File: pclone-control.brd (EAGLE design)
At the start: 72.4 x 68.6 mm, 20 parts

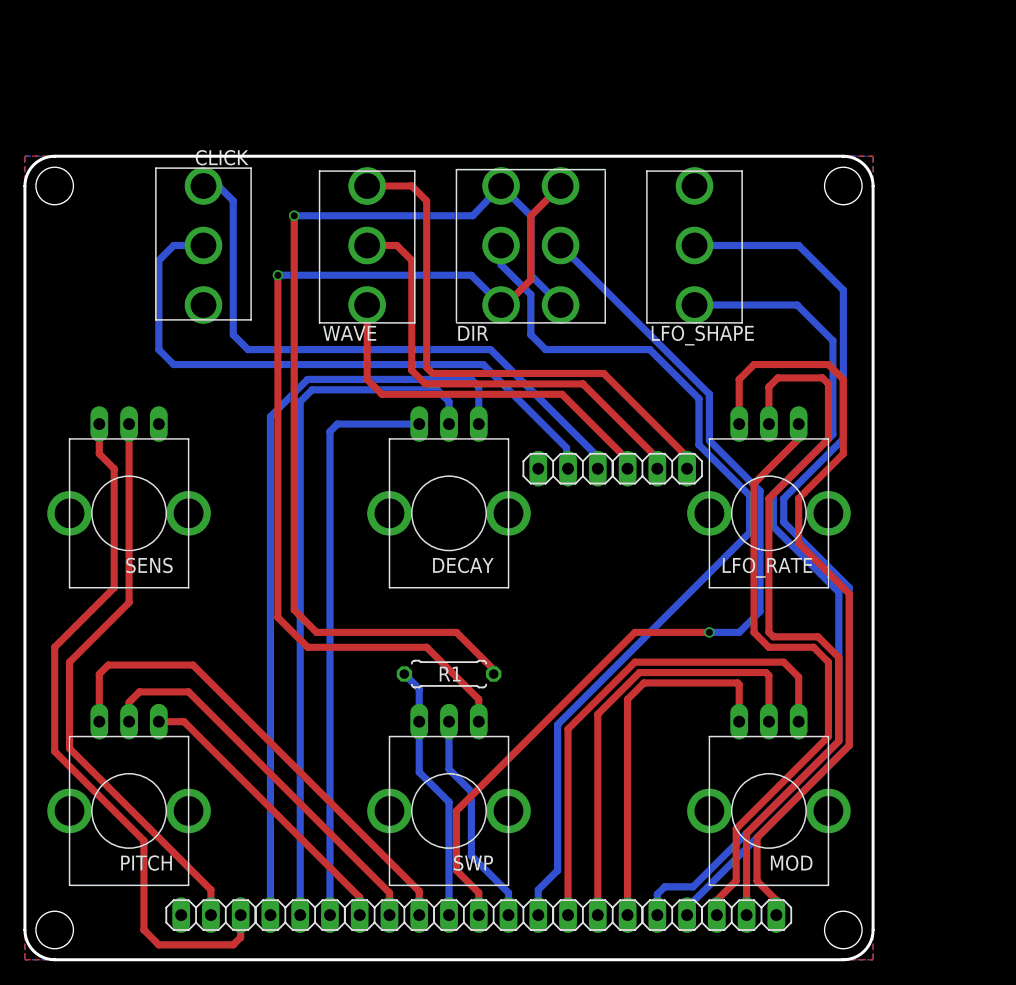
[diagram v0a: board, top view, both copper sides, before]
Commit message: work in progress
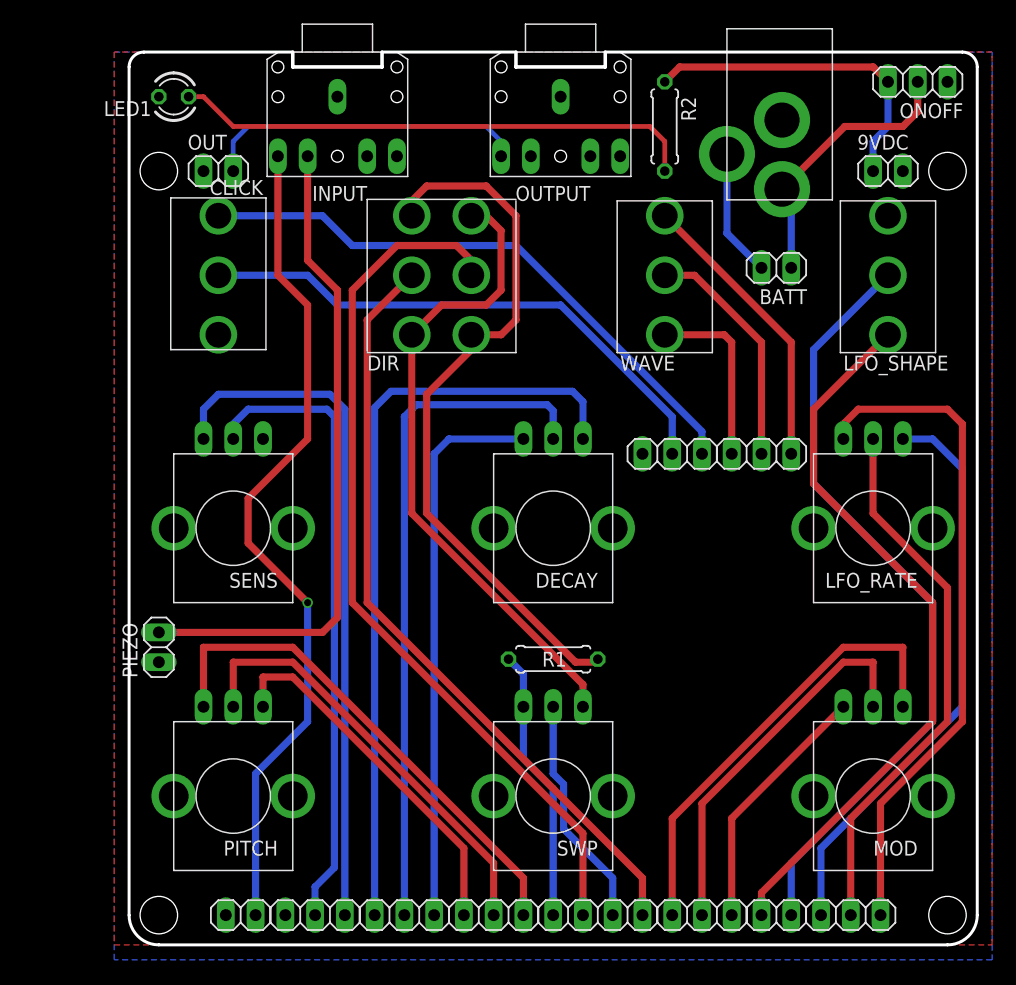
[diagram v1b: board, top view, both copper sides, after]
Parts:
- added 9VDC, BATT, IN, OUT, PIEZO: (no value), pinhead:1X02
- added INPUT, OUTPUT: TRUCONNECTJACK, jason_eagle6:TRUCONNECTJACK
- added LED1: (no value), led:LED3MM
- added ONOFF: (no value), pinhead:1X03
- added R2: 4k7, rcl:0207/7
- added U$4: 2.1MMJACKTHM, adafruit:PJ-102A
- moved WAVE 25.5 mm to (54.6, 58.4)
- moved LFO_SHAPE 16.7 mm to (73.7, 58.4)
- moved DECAY 8.98 mm to (45.1, 36.8)
- moved J8 8.98 mm to (55.2, 43.2)
- moved J9 8.98 mm to (62.9, 43.2)
- moved LFO_RATE 8.98 mm to (72.4, 36.8)
- moved MOD 8.98 mm to (72.4, 14.0)
- moved PITCH 8.98 mm to (17.8, 14.0)
- moved R1 8.98 mm to (45.1, 25.7)
- moved SENS 8.98 mm to (17.8, 36.8)
- moved SWP 8.98 mm to (45.1, 14.0)
- moved J6 8.89 mm to (64.1, 3.81)
- moved J3 8.89 mm to (40.0, 3.81)
- moved J1 8.89 mm to (24.8, 3.81)
- moved J4 8.89 mm to (48.9, 3.81)
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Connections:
- new net N$15: BATT.1, ONOFF.2, U$4.TIP
- new net N$29: BATT.2, U$4.RING_SW
- new net N$30: 9VDC.1, ONOFF.3, R2.1
- new net N$31: LED1.A, R2.2
- new net N$32: OUT.2, OUTPUT.TIP
- new net N$33: INPUT.TIP_NC, PIEZO.2
- new net N$34: IN.2, INPUT.TIP
- net GND: now also 9VDC.2, IN.1, INPUT.RING, INPUT.RING_NC, INPUT.SLEEVE, LED1.K, OUT.1, OUTPUT.RING, OUTPUT.RING_NC, OUTPUT.SLEEVE, PIEZO.1, U$4.RING
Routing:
- net N$34: track 0.00 -> 71.9 mm, vias 0 -> 1
- net N$33: track 0.00 -> 56.2 mm
- net N$31: track 0.00 -> 44.8 mm
- net N$3: track 83.7 -> 55.1 mm, vias 1 -> 0
- net N$30: track 0.00 -> 28.2 mm
- net N$32: track 0.00 -> 27.7 mm
- net N$15: track 0.00 -> 23.9 mm
- net N$2: track 84.2 -> 61.8 mm, vias 1 -> 0
- net N$8: track 46.2 -> 24.8 mm
- net N$9: track 38.7 -> 20.1 mm
- net N$26: track 64.2 -> 46.7 mm
- net N$7: track 32.2 -> 15.5 mm
- net N$4: track 78.6 -> 65.9 mm
- net N$12: track 74.3 -> 62.4 mm
- net N$13: track 77.8 -> 66.4 mm
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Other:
- board size 72.4 x 68.6 mm -> 72.4 x 76.2 mm
